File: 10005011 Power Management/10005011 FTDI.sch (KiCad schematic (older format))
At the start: 49 parts, among them IC11 TPS5430DDA, IC12 LM4120AIM5-3.0, IC26 NC7SZ66, IC27 NC7SZ66, IC4 FT2232, IC8 LF33CDT, J1 USB Mini B, Q1 6 MHz

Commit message: Powermanagement dev netlist fix
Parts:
- C44: symbol Device:CP -> 10005011_Power_Management:CP
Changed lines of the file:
@@
 	15650 4200 15650 4300
 $Comp
-L Device:CP C44
+L 10005011_Power_Management:CP C44
 U 1 1 5EFB991E
 P 14200 4550
@@
 Connection ~ 13850 1850
 $Comp
-L 10005011_Power_Management:0VANA #PWR?
+L 10005011_Power_Management:0VANA #PWR0186
 U 1 1 5EA51CD6
 P 11850 8800
-F 0 "#PWR?" H 11850 8550 50  0001 C CNN
+F 0 "#PWR0186" H 11850 8550 50  0001 C CNN
 F 1 "0VANA" H 11855 8627 50  0000 C CNN
 F 2 "" H 11850 8800 50  0001 C CNN
@@
 $EndComp
 $Comp
-L 10005011_Power_Management:0VANA #PWR?
+L 10005011_Power_Management:0VANA #PWR0187
 U 1 1 5EA54662
 P 13850 8750
-F 0 "#PWR?" H 13850 8500 50  0001 C CNN
+F 0 "#PWR0187" H 13850 8500 50  0001 C CNN
 F 1 "0VANA" H 13855 8577 50  0000 C CNN
 F 2 "" H 13850 8750 50  0001 C CNN

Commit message: Powermanagement dev library
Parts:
- C55: Description (none) -> CAPACITOR CERAMIC, 100NF, +/-10%, 50V, X7R,0805; Item Number (none) -> 10022135
- D11: footprint 10005011 Power Management:SMB_1 -> Diode_SMD:D_SMB; symbol 10005011_Power_Management_Schematic_Symbols:STPS340U -> 10005011_Power_Management:STPS340U; Description DIODE SCHOTTKY 40V 3A SMB -> DIODE SCHOTTKY, 3A, 40V; Item Number (none) -> 10022656; Manufacturer (none) -> STMICROELECTRONICS; Manufacturer_No (none) -> STPS340U; Mfgr STMicroelectronics -> (none); Mfgr_PN STPS340U -> (none)
- D16: BOM_Footprint SOT23 -> (none); Item Number (none) -> 10022653
- IC12: symbol page3:LM4120AIM5-3.0 -> 10005011_Power_Management:LM4120AIM5-3.0; Description (none) -> IC,VOLTAGE REFERENCE,5MA,3V +/-2%,SOT23; Item Number (none) -> 10022896; MNF TI -> (none); MNF PN LM4120AIM5-3.0 -> (none); Manufacturer (none) -> NATIONAL SEMICONDUCTOR; Manufacturer_No (none) -> LM4120AIM5-3.0/NOPB
- IC26, IC27: symbol page3:NC7SZ66 -> 10005011_Power_Management:NC7SZ66; Description (none) -> IC,BUS SWITCH,SC70; Item Number (none) -> 10039588; Manufacturer (none) -> FAIRCHILD SEMICONDUCTOR; Manufacturer_No (none) -> NC7SZ66P5X
- J1: symbol page3:USB_B_Mini_2shield -> 10005011_Power_Management:USB_B_Mini_2shield; Description (none) -> USB MINI B; Item Number (none) -> 10022867; Manufacturer (none) -> MOLEX; Manufacturer_No (none) -> 54819-0519
- L1: symbol 10005011_Power_Management_Schematic_Symbols:MH2029-221Y -> Device:Ferrite_Bead_Small
- L7: symbol 10005011_Power_Management_Schematic_Symbols:MH2029-221Y -> Device:Ferrite_Bead_Small; Bom_Footprint 0805 -> (none); Item Number (none) -> 10039587
- L8: symbol page3:Common_Mode_Choke -> 10005011_Power_Management:DLP31SN551ML2L; Description (none) -> COMMON MODE CHOKE COIL 550OHM; Item Number (none) -> 10039588; Manufacturer (none) -> MURATA; Manufacturer_No (none) -> DLP31SN551ML2L
- ML1: symbol 10005011_Power_Management_Schematic_Symbols:B72500T0040M060 -> Device:Varistor; Bom_Footprint 0603 -> (none); Description VARISTOR 8V 30A 0603 -> SMD VARISTOR, 5.5V,C0603; Item Number (none) -> 10022926
- PG1, PG2: symbol 10005011_Power_Management_Schematic_Symbols:82356050050 -> Device:D_TVS; Description ESD SUPPRESSOR 0603; 5VDC; 5PF -> VARISTOR, CMS PROTECTION ESD SURGE SUPPRESSOR,C0603; Item Number (none) -> 10022946
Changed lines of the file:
@@
 F 4 "Yageo" H 10150 5050 50  0001 C CNN "Mnf"
 F 5 "223858055649" H 10150 5050 50  0001 C CNN "Mnf PN"
+F 6 "CAPACITOR CERAMIC, 100NF, +/-10%, 50V, X7R,0805" H 10150 5050 50  0001 C CNN "Description"
+F 7 "10022135" H 10150 5050 50  0001 C CNN "Item Number"
 	1    10150 5050
 	-1   0    0    1
@@
 	6200 2050 6100 2050
 $Comp
-L 10005011_Power_Management_Schematic_Symbols:82356050050 PG2
+L Device:D_TVS PG2
 U 1 1 5F152259
 P 2000 3700
@@
 F 6 "Digi-Key" H 2000 3700 50  0001 C CNN "Source"
 F 7 "732-13295-1-ND" H 2000 3700 50  0001 C CNN "Source_PN"
-F 8 "ESD SUPPRESSOR 0603; 5VDC; 5PF" H 2000 3700 50  0001 C CNN "Description"
+F 8 "VARISTOR, CMS PROTECTION ESD SURGE SUPPRESSOR,C0603" H 2000 3700 50  0001 C CNN "Description"
+F 9 "10022946" H 2000 3700 50  0001 C CNN "Item Number"
 	1    2000 3700
 	0    1    -1   0
@@
 $EndComp
 $Comp
-L page3:USB_B_Mini_2shield J1
+L 10005011_Power_Management:USB_B_Mini_2shield J1
 U 1 1 5F15225D
 P 1350 3350
@@
 F 1 "USB Mini B" V 1100 3100 50  0000 L CNN
 F 2 "10005011 Power Management:MOL54819-0511_1" H 1600 3500 50  0001 C CNN
-F 3 "https://www.molex.com/molex/products/part-detail/io_connectors/0548190519" H 1600 3500 50  0001 C CNN
+F 3 "~" H 1600 3500 50  0001 C CNN
+F 4 "USB MINI B" H 1350 3350 50  0001 C CNN "Description"
+F 5 "10022867" H 1350 3350 50  0001 C CNN "Item Number"
+F 6 "MOLEX" H 1350 3350 50  0001 C CNN "Manufacturer"
+F 7 "54819-0519" H 1350 3350 50  0001 C CNN "Manufacturer_No"
 	1    1350 3350
 	1    0    0    -1
 $EndComp
 $Comp
-L 10005011_Power_Management_Schematic_Symbols:MH2029-221Y L7
+L Device:Ferrite_Bead_Small L7
 U 1 1 5EC7397A
 P 1650 4050
@@
 F 7 "Digi-Key" H 1650 4050 50  0001 C CNN "Source"
 F 8 "MH2029-221YTR-ND" H 1650 4050 50  0001 C CNN "Source_PN"
-F 9 "0805" V 1986 4050 62  0001 C CNN "Bom_Footprint"
+F 9 "10039587" V 1650 4050 50  0001 C CNN "Item Number"
 	1    1650 4050
 	0    -1   1    0
 $EndComp
 $Comp
-L 10005011_Power_Management_Schematic_Symbols:MH2029-221Y L1
+L Device:Ferrite_Bead_Small L1
 U 1 1 5F15225F
 P 2700 1700
@@
 $EndComp
 $Comp
-L 10005011_Power_Management_Schematic_Symbols:B72500T0040M060 ML1
+L Device:Varistor ML1
 U 1 1 5F152260
 P 3300 3700
@@
 F 6 "TDK Electronics Inc." H 3300 3700 50  0001 C CNN "Mfgr"
 F 7 "B72500T0040M060" H 3300 3700 50  0001 C CNN "Mfgr_PN"
-F 8 "VARISTOR 8V 30A 0603" H 3300 3700 50  0001 C CNN "Description"
-F 9 "0603" H 3179 3791 50  0001 R CNN "Bom_Footprint"
+F 8 "SMD VARISTOR, 5.5V,C0603" H 3300 3700 50  0001 C CNN "Description"
+F 9 "" H 3179 3791 50  0001 R CNN "Bom_Footprint"
+F 10 "10022926" H 3300 3700 50  0001 C CNN "Item Number"
 	1    3300 3700
 	-1   0    0    1
@@
 	2650 3550 2650 3450
 $Comp
-L 10005011_Power_Management_Schematic_Symbols:82356050050 PG1
+L Device:D_TVS PG1
 U 1 1 5EC6C643
 P 2650 3700
@@
 F 6 "Digi-Key" H 2650 3700 50  0001 C CNN "Source"
 F 7 "732-13295-1-ND" H 2650 3700 50  0001 C CNN "Source_PN"
-F 8 "ESD SUPPRESSOR 0603; 5VDC; 5PF" H 2650 3700 50  0001 C CNN "Description"
+F 8 "VARISTOR, CMS PROTECTION ESD SURGE SUPPRESSOR,C0603" H 2650 3700 50  0001 C CNN "Description"
+F 9 "10022946" H 2650 3700 50  0001 C CNN "Item Number"
 	1    2650 3700
 	0    1    -1   0
@@
 $EndComp
 $Comp
-L page3:Common_Mode_Choke L8
+L 10005011_Power_Management:DLP31SN551ML2L L8
 U 1 1 5ECE0914
 P 3950 3250
@@
 F 2 "10005011 Power Management:DLP31S-AIROX_1" H 3950 3290 50  0001 C CNN
 F 3 "https://www.murata.com/en-eu/products/productdata/8796756410398/EFLE0007.pdf" H 3950 3290 50  0001 C CNN
+F 4 "COMMON MODE CHOKE COIL 550OHM" H 3950 3250 50  0001 C CNN "Description"
+F 5 "10039588" H 3950 3250 50  0001 C CNN "Item Number"
+F 6 "MURATA" H 3950 3250 50  0001 C CNN "Manufacturer"
+F 7 "DLP31SN551ML2L" H 3950 3250 50  0001 C CNN "Manufacturer_No"
 	1    3950 3250
 	1    0    0    -1
@@
 	12800 4300 12800 4400
 $Comp
-L 10005011_Power_Management_Schematic_Symbols:STPS340U D11
+L 10005011_Power_Management:STPS340U D11
 U 1 1 5EE9F24C
 P 13400 4650
 F 0 "D11" V 13354 4729 50  0000 L CNN
 F 1 "STPS340U" V 13445 4729 50  0000 L CNN
-F 2 "10005011 Power Management:SMB_1" H 13400 4650 50  0001 C CNN
+F 2 "Diode_SMD:D_SMB" H 13400 4650 50  0001 C CNN
 F 3 "http://www.st.com/content/ccc/resource/technical/document/datasheet/bb/db/21/0c/04/d9/41/a5/CD00000844.pdf/files/CD00000844.pdf/jcr:content/translations/en.CD00000844.pdf" H 13400 4650 50  0001 C CNN
-F 4 "STMicroelectronics" H 13400 4650 50  0001 C CNN "Mfgr"
-F 5 "STPS340U" H 13400 4650 50  0001 C CNN "Mfgr_PN"
-F 6 "Digi-Key" H 13400 4650 50  0001 C CNN "Source"
-F 7 "497-2465-1-ND" H 13400 4650 50  0001 C CNN "Source_PN"
-F 8 "DIODE SCHOTTKY 40V 3A SMB" H 13400 4650 50  0001 C CNN "Description"
+F 4 "Digi-Key" H 13400 4650 50  0001 C CNN "Source"
+F 5 "497-2465-1-ND" H 13400 4650 50  0001 C CNN "Source_PN"
+F 6 "DIODE SCHOTTKY, 3A, 40V" H 13400 4650 50  0001 C CNN "Description"
+F 7 "10022656" H 13400 4650 50  0001 C CNN "Item Number"
+F 8 "STMICROELECTRONICS" H 13400 4650 50  0001 C CNN "Manufacturer"
+F 9 "STPS340U" H 13400 4650 50  0001 C CNN "Manufacturer_No"
 	1    13400 4650
 	0    1    1    0
@@
 5V REGULATOR
 $Comp
-L page3:LM4120AIM5-3.0 IC12
+L 10005011_Power_Management:LM4120AIM5-3.0 IC12
 U 1 1 5F0C731D
 P 12375 8350
-F 0 "IC12" H 12100 8700 50  0000 L CNN
-F 1 "LM4120AIM5-3.0" H 12075 8000 50  0000 L CNN
+F 0 "IC12" H 12375 8817 50  0000 C CNN
+F 1 "LM4120AIM5-3.0" H 12375 8726 50  0000 C CNN
 F 2 "10005011 Power Management:SOT23-5_1" H 12075 7850 50  0001 L CIN
 F 3 "http://www.ti.com/lit/ds/symlink/lm4120.pdf" H 12975 7750 50  0001 C CIN
-F 4 "TI" H 12375 7775 50  0001 C CNN "MNF"
-F 5 "LM4120AIM5-3.0" H 12400 7925 50  0001 C CNN "MNF PN"
+F 4 "IC,VOLTAGE REFERENCE,5MA,3V +/-2%,SOT23" H 12375 7775 50  0001 C CNN "Description"
+F 5 "10022896" H 12400 7925 50  0001 C CNN "Item Number"
+F 6 "NATIONAL SEMICONDUCTOR" H 12375 8350 50  0001 C CNN "Manufacturer"
+F 7 "LM4120AIM5-3.0/NOPB" H 12375 8350 50  0001 C CNN "Manufacturer_No"
 	1    12375 8350
 	1    0    0    -1
@@
 F 2 "10005011 Power Management:SOT23-1G_1" H 7225 1675 50  0001 L CNN
 F 3 "https://media.digikey.com/pdf/Data%20Sheets/ON%20Semiconductor%20PDFs/BAT54(A,C,S).pdf" H 7420 2250 50  0001 C CNN
-F 4 "SOT23" H 7450 2383 50  0001 C CNN "BOM_Footprint"
-F 5 "DIODE ARRAY SCHOTTKY 30V SOT23-3" H 7825 1975 60  0001 C CNN "Description"
-F 6 "ON Semiconductor" H 7825 1975 60  0001 C CNN "Mfgr"
-F 7 "BAT54C" H 7825 1975 60  0001 C CNN "Mfgr_PN"
-F 8 "Digi-Key" H 7675 1975 60  0001 C CNN "Source"
-F 9 "BAT54CFSCT-ND" H 7650 1975 60  0001 C CNN "Source_PN"
+F 4 "DIODE ARRAY SCHOTTKY 30V SOT23-3" H 7825 1975 60  0001 C CNN "Description"
+F 5 "ON Semiconductor" H 7825 1975 60  0001 C CNN "Mfgr"
+F 6 "BAT54C" H 7825 1975 60  0001 C CNN "Mfgr_PN"
+F 7 "Digi-Key" H 7675 1975 60  0001 C CNN "Source"
+F 8 "BAT54CFSCT-ND" H 7650 1975 60  0001 C CNN "Source_PN"
+F 9 "10022653" H 7500 2150 50  0001 C CNN "Item Number"
 	1    7500 2150
 	1    0    0    -1
@@
 V-USB
 $Comp
-L page3:NC7SZ66 IC26
+L 10005011_Power_Management:NC7SZ66 IC26
 U 1 1 5F152257
 P 8000 4250
 F 0 "IC26" H 7750 4500 50  0000 L CNN
-F 1 "NC7SZ66" H 8000 4000 50  0000 L CNN
+F 1 "NC7SZ66" H 8050 4500 50  0000 L CNN
 F 2 "10005011 Power Management:SC70-5_1" H 8000 4050 50  0001 C CNN
 F 3 "https://www.onsemi.com/pub/Collateral/NC7SZ66-D.pdf" H 7350 4850 50  0001 C CNN
+F 4 "IC,BUS SWITCH,SC70" H 8000 4250 50  0001 C CNN "Description"
+F 5 "10039588" H 8000 4250 50  0001 C CNN "Item Number"
+F 6 "FAIRCHILD SEMICONDUCTOR" H 8000 4250 50  0001 C CNN "Manufacturer"
+F 7 "NC7SZ66P5X" H 8000 4250 50  0001 C CNN "Manufacturer_No"
 	1    8000 4250
 	1    0    0    -1
 $EndComp
 $Comp
-L page3:NC7SZ66 IC27
+L 10005011_Power_Management:NC7SZ66 IC27
 U 1 1 5F152256
 P 7750 3050
@@
 F 2 "10005011 Power Management:SC70-5_1" H 7750 2850 50  0001 C CNN
 F 3 "https://www.onsemi.com/pub/Collateral/NC7SZ66-D.pdf" H 7100 3650 50  0001 C CNN
+F 4 "IC,BUS SWITCH,SC70" H 7750 3050 50  0001 C CNN "Description"
+F 5 "10039588" H 7750 3050 50  0001 C CNN "Item Number"
+F 6 "FAIRCHILD SEMICONDUCTOR" H 7750 3050 50  0001 C CNN "Manufacturer"
+F 7 "NC7SZ66P5X" H 7750 3050 50  0001 C CNN "Manufacturer_No"
 	1    7750 3050
 	1    0    0    -1

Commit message: fix D11 footprint and library
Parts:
- D11: footprint Diode_SMD:D_SMB -> 10005011 Power Management:SMB_1
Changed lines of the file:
@@
 F 0 "D11" V 13354 4729 50  0000 L CNN
 F 1 "STPS340U" V 13445 4729 50  0000 L CNN
-F 2 "Diode_SMD:D_SMB" H 13400 4650 50  0001 C CNN
+F 2 "10005011 Power Management:SMB_1" H 13400 4650 50  0001 C CNN
 F 3 "http://www.st.com/content/ccc/resource/technical/document/datasheet/bb/db/21/0c/04/d9/41/a5/CD00000844.pdf/files/CD00000844.pdf/jcr:content/translations/en.CD00000844.pdf" H 13400 4650 50  0001 C CNN
 F 4 "Digi-Key" H 13400 4650 50  0001 C CNN "Source"

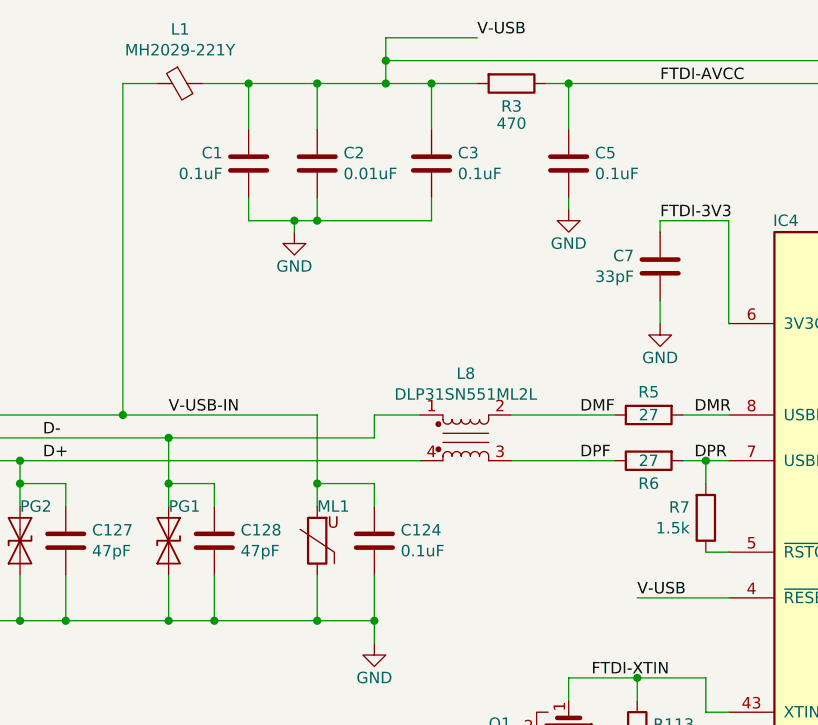
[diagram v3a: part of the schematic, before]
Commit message: item 10022607
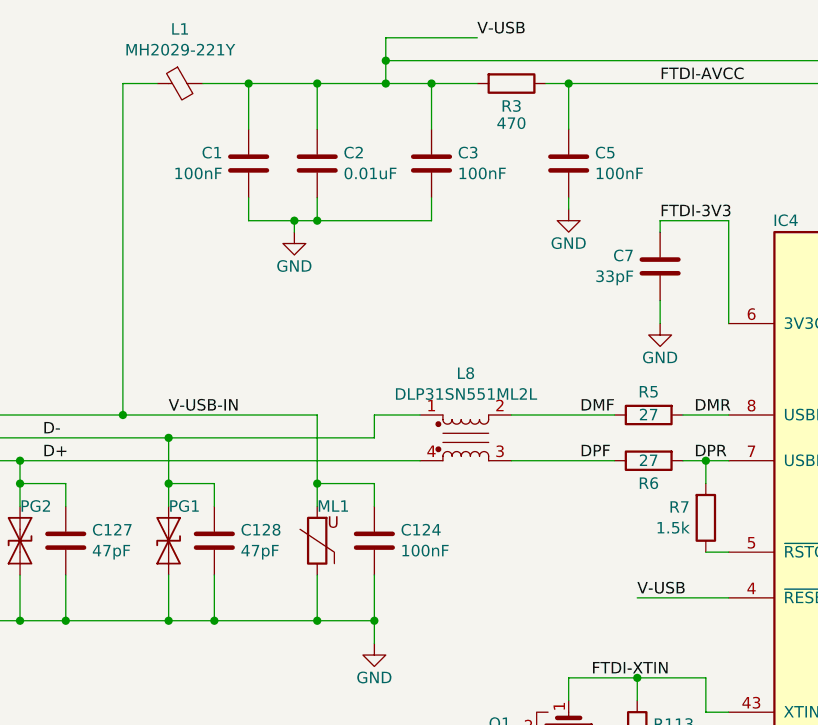
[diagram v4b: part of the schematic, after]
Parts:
- C1, C124, C3, C5: value 0.1uF -> 100nF; Bom_Footprint 0402 -> (none); Description CAP CER 47PF 50V C0G/NP0 0402 -> CAPACITOR,100NF,16V,+/-10%,X7R,0402; Item Number (none) -> 10022607; Manufacturer (none) -> MURATA; Manufacturer_No (none) -> GRM155R71C104JA88J
- C126, C35, C36, C46, C58, C59: Description (none) -> CAPACITOR,100NF,16V,+/-10%,X7R,0402; Item Number (none) -> 10022607; Manufacturer (none) -> MURATA; Manufacturer_No (none) -> GRM155R71C104JA88J
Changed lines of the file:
@@
 F 4 "Murata" H 15150 4550 50  0001 C CNN "Mnf"
 F 5 "GRM155R71C104JA88J" H 15150 4550 50  0001 C CNN "Mnf PN"
+F 6 "CAPACITOR,100NF,16V,+/-10%,X7R,0402" H 15150 4550 50  0001 C CNN "Description"
+F 7 "10022607" H 15150 4550 50  0001 C CNN "Item Number"
+F 8 "MURATA" H 15150 4550 50  0001 C CNN "Manufacturer"
+F 9 "GRM155R71C104JA88J" H 15150 4550 50  0001 C CNN "Manufacturer_No"
 	1    15150 4550
 	1    0    0    -1
@@
 F 4 "Murata" H 11400 8500 50  0001 C CNN "Mnf"
 F 5 "GRM155R71C104JA88J" H 11400 8500 50  0001 C CNN "Mnf PN"
+F 6 "CAPACITOR,100NF,16V,+/-10%,X7R,0402" H 11400 8500 50  0001 C CNN "Description"
+F 7 "10022607" H 11400 8500 50  0001 C CNN "Item Number"
+F 8 "MURATA" H 11400 8500 50  0001 C CNN "Manufacturer"
+F 9 "GRM155R71C104JA88J" H 11400 8500 50  0001 C CNN "Manufacturer_No"
 	1    11400 8500
 	1    0    0    1
@@
 F 4 "Murata" H 13850 8400 50  0001 C CNN "Mnf"
 F 5 "GRM155R71C104JA88J" H 13850 8400 50  0001 C CNN "Mnf PN"
+F 6 "CAPACITOR,100NF,16V,+/-10%,X7R,0402" H 13850 8400 50  0001 C CNN "Description"
+F 7 "10022607" H 13850 8400 50  0001 C CNN "Item Number"
+F 8 "MURATA" H 13850 8400 50  0001 C CNN "Manufacturer"
+F 9 "GRM155R71C104JA88J" H 13850 8400 50  0001 C CNN "Manufacturer_No"
 	1    13850 8400
 	1    0    0    -1
@@
 P 3000 2050
 F 0 "C1" H 3114 2004 50  0000 L CNN
-F 1 "0.1uF" H 3114 2095 50  0000 L CNN
+F 1 "100nF" H 3114 2095 50  0000 L CNN
 F 2 "10005011 Power Management:C0402_1" H 3038 1900 50  0001 C CNN
 F 3 "https://psearch.en.murata.com/capacitor/product/GCM155R71C104KA55%23.pdf" H 3000 2050 50  0001 C CNN
@@
 F 6 "Digi-Key" H 3000 2050 50  0001 C CNN "Source"
 F 7 "490-7998-1-ND" H 3000 2050 50  0001 C CNN "Source_PN"
-F 8 "0402" H 2885 2095 50  0001 R CNN "Bom_Footprint"
-F 9 "CAP CER 47PF 50V C0G/NP0 0402" H 3000 2050 50  0001 C CNN "Description"
+F 8 "" H 2885 2095 50  0001 R CNN "Bom_Footprint"
+F 9 "CAPACITOR,100NF,16V,+/-10%,X7R,0402" H 3000 2050 50  0001 C CNN "Description"
 F 10 "X7R" H 3000 2050 50  0001 C CNN "Dielectric"
 F 11 "16V" H 2885 2186 50  0001 R CNN "Voltage"
+F 12 "10022607" H 3000 2050 50  0001 C CNN "Item Number"
+F 13 "MURATA" H 3000 2050 50  0001 C CNN "Manufacturer"
+F 14 "GRM155R71C104JA88J" H 3000 2050 50  0001 C CNN "Manufacturer_No"
 	1    3000 2050
 	-1   0    0    1
@@
 P 3800 2050
 F 0 "C3" H 3685 2004 50  0000 R CNN
-F 1 "0.1uF" H 3685 2095 50  0000 R CNN
+F 1 "100nF" H 3685 2095 50  0000 R CNN
 F 2 "10005011 Power Management:C0402_1" H 3838 1900 50  0001 C CNN
 F 3 "https://psearch.en.murata.com/capacitor/product/GCM155R71C104KA55%23.pdf" H 3800 2050 50  0001 C CNN
@@
 F 6 "Digi-Key" H 3800 2050 50  0001 C CNN "Source"
 F 7 "490-7998-1-ND" H 3800 2050 50  0001 C CNN "Source_PN"
-F 8 "0402" H 3685 2095 50  0001 R CNN "Bom_Footprint"
-F 9 "CAP CER 47PF 50V C0G/NP0 0402" H 3800 2050 50  0001 C CNN "Description"
+F 8 "" H 3685 2095 50  0001 R CNN "Bom_Footprint"
+F 9 "CAPACITOR,100NF,16V,+/-10%,X7R,0402" H 3800 2050 50  0001 C CNN "Description"
 F 10 "X7R" H 3800 2050 50  0001 C CNN "Dielectric"
 F 11 "16V" H 3685 2186 50  0001 R CNN "Voltage"
+F 12 "10022607" H 3800 2050 50  0001 C CNN "Item Number"
+F 13 "MURATA" H 3800 2050 50  0001 C CNN "Manufacturer"
+F 14 "GRM155R71C104JA88J" H 3800 2050 50  0001 C CNN "Manufacturer_No"
 	1    3800 2050
 	-1   0    0    1
@@
 P 3550 3700
 F 0 "C124" H 3665 3746 50  0000 L CNN
-F 1 "0.1uF" H 3665 3655 50  0000 L CNN
+F 1 "100nF" H 3665 3655 50  0000 L CNN
 F 2 "10005011 Power Management:C0402_1" H 3588 3550 50  0001 C CNN
 F 3 "https://psearch.en.murata.com/capacitor/product/GCM155R71C104KA55%23.pdf" H 3550 3700 50  0001 C CNN
@@
 F 6 "Digi-Key" H 3550 3700 50  0001 C CNN "Source"
 F 7 "490-7998-1-ND" H 3550 3700 50  0001 C CNN "Source_PN"
-F 8 "0402" H 3665 3655 50  0001 L CNN "Bom_Footprint"
-F 9 "CAP CER 47PF 50V C0G/NP0 0402" H 3550 3700 50  0001 C CNN "Description"
+F 8 "" H 3665 3655 50  0001 L CNN "Bom_Footprint"
+F 9 "CAPACITOR,100NF,16V,+/-10%,X7R,0402" H 3550 3700 50  0001 C CNN "Description"
 F 10 "X7R" H 3550 3700 50  0001 C CNN "Dielectric"
 F 11 "16V" H 3665 3564 50  0001 L CNN "Voltage"
+F 12 "10022607" H 3550 3700 50  0001 C CNN "Item Number"
+F 13 "MURATA" H 3550 3700 50  0001 C CNN "Manufacturer"
+F 14 "GRM155R71C104JA88J" H 3550 3700 50  0001 C CNN "Manufacturer_No"
 	1    3550 3700
 	1    0    0    -1
@@
 P 4400 2050
 F 0 "C5" H 4515 2096 50  0000 L CNN
-F 1 "0.1uF" H 4515 2005 50  0000 L CNN
+F 1 "100nF" H 4515 2005 50  0000 L CNN
 F 2 "10005011 Power Management:C0402_1" H 4438 1900 50  0001 C CNN
 F 3 "https://psearch.en.murata.com/capacitor/product/GCM155R71C104KA55%23.pdf" H 4400 2050 50  0001 C CNN
@@
 F 6 "Digi-Key" H 4400 2050 50  0001 C CNN "Source"
 F 7 "490-7998-1-ND" H 4400 2050 50  0001 C CNN "Source_PN"
-F 8 "0402" H 4515 2005 50  0001 L CNN "Bom_Footprint"
-F 9 "CAP CER 47PF 50V C0G/NP0 0402" H 4400 2050 50  0001 C CNN "Description"
+F 8 "" H 4515 2005 50  0001 L CNN "Bom_Footprint"
+F 9 "CAPACITOR,100NF,16V,+/-10%,X7R,0402" H 4400 2050 50  0001 C CNN "Description"
 F 10 "X7R" H 4400 2050 50  0001 C CNN "Dielectric"
 F 11 "16V" H 4515 1914 50  0001 L CNN "Voltage"
+F 12 "10022607" H 4400 2050 50  0001 C CNN "Item Number"
+F 13 "MURATA" H 4400 2050 50  0001 C CNN "Manufacturer"
+F 14 "GRM155R71C104JA88J" H 4400 2050 50  0001 C CNN "Manufacturer_No"
 	1    4400 2050
 	1    0    0    -1
@@
 F 2 "10005011 Power Management:C0402_1" H 12638 1950 50  0001 C CNN
 F 3 "~" H 12600 2100 50  0001 C CNN
+F 4 "CAPACITOR,100NF,16V,+/-10%,X7R,0402" H 12600 2100 50  0001 C CNN "Description"
+F 5 "10022607" H 12600 2100 50  0001 C CNN "Item Number"
+F 6 "MURATA" H 12600 2100 50  0001 C CNN "Manufacturer"
+F 7 "GRM155R71C104JA88J" H 12600 2100 50  0001 C CNN "Manufacturer_No"
 	1    12600 2100
 	1    0    0    1
@@
 F 2 "10005011 Power Management:C0402_1" H 11638 1950 50  0001 C CNN
 F 3 "~" H 11600 2100 50  0001 C CNN
+F 4 "CAPACITOR,100NF,16V,+/-10%,X7R,0402" H 11600 2100 50  0001 C CNN "Description"
+F 5 "10022607" H 11600 2100 50  0001 C CNN "Item Number"
+F 6 "MURATA" H 11600 2100 50  0001 C CNN "Manufacturer"
+F 7 "GRM155R71C104JA88J" H 11600 2100 50  0001 C CNN "Manufacturer_No"
 	1    11600 2100
 	1    0    0    1
@@
 F 2 "10005011 Power Management:C0402_1" H 8788 3350 50  0001 C CNN
 F 3 "~" H 8750 3500 50  0001 C CNN
+F 4 "CAPACITOR,100NF,16V,+/-10%,X7R,0402" H 8750 3500 50  0001 C CNN "Description"
+F 5 "10022607" H 8750 3500 50  0001 C CNN "Item Number"
+F 6 "MURATA" H 8750 3500 50  0001 C CNN "Manufacturer"
+F 7 "GRM155R71C104JA88J" H 8750 3500 50  0001 C CNN "Manufacturer_No"
 	1    8750 3500
 	-1   0    0    1
